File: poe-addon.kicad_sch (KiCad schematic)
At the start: 16 parts, among them U1 25AA02E48T-I_OT, X1 ARJM11-104, X2 Conn_01x05_Male, X3 Conn_01x05_Male

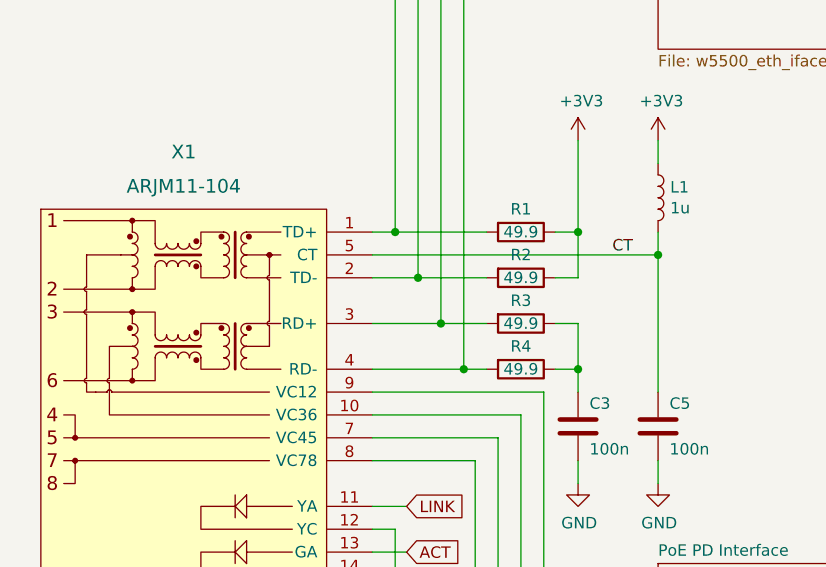
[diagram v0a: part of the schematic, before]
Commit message: Add LCSC part numbers
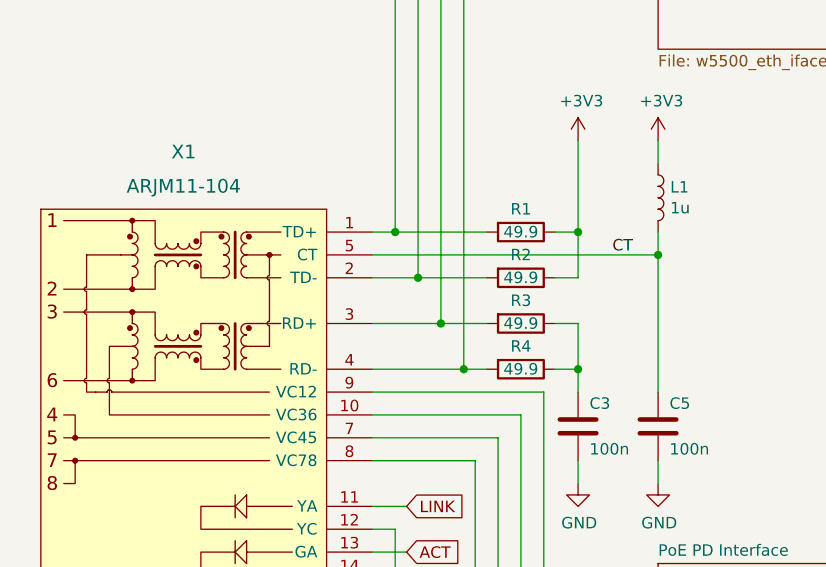
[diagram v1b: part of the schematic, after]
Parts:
- U1: LCSC (none) -> C145570
